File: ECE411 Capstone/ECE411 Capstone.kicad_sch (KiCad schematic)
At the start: 27 parts, among them SW1 SW_Push, SW2 SW_Push, SW3 SW_Push, SW4 SW_Push, SW5 SW_Push, SW6 SW_Push, SW7 SW_Push, U1 IS31FL3218-GR

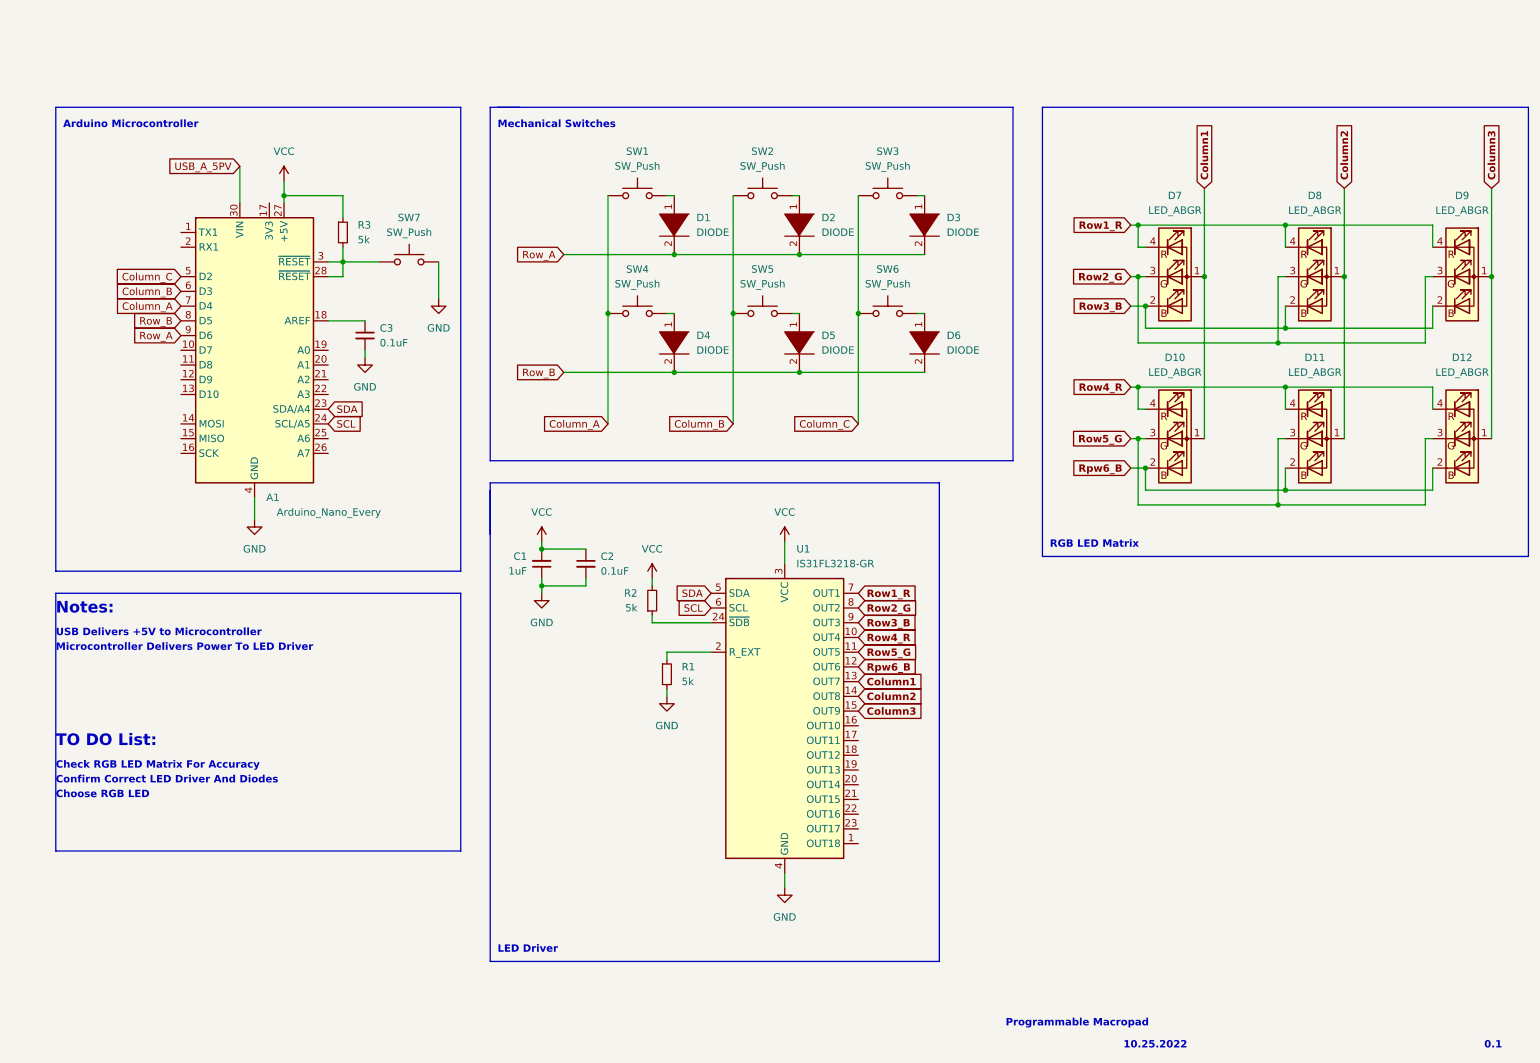
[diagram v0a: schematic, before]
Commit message: Updated Schematic + PCB for review
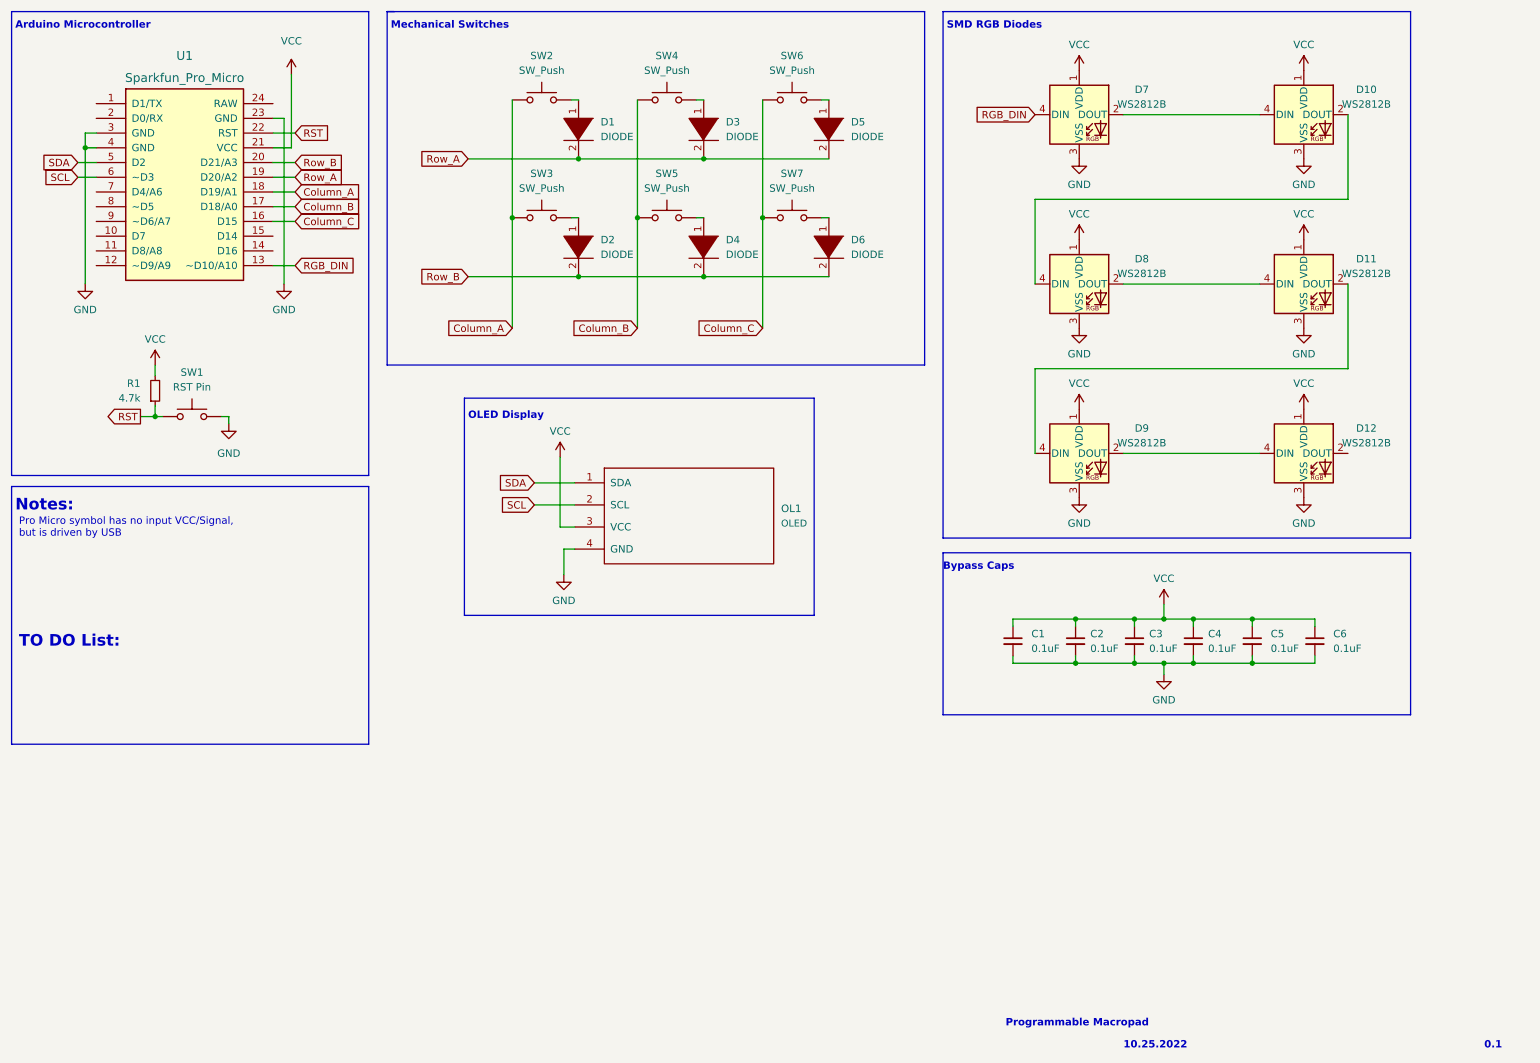
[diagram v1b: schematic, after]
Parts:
- removed A1: Arduino_Nano_Every, Module:Arduino_Nano, symbol MCU_Module:Arduino_Nano_Every
- removed D10, D11, D12, D7, D8, D9: LED_ABGR, symbol Device:LED_ABGR
- removed R2, R3: 5k, symbol Device:R_Small
- removed SW7: SW_Push, symbol Switch:SW_Push
- removed U1: IS31FL3218-GR, Package_SO:SOP-24_7.5x15.4mm_P1.27mm, symbol Driver_LED:IS31FL3218-GR
- added C4, C5, C6: 0.1uF, Capacitor_SMD:C_01005_0402Metric, symbol Device:C_Small
- added D10, D11, D12, D7, D8, D9: WS2812B, LED_SMD:LED_WS2812B_PLCC4_5.0x5.0mm_P3.2mm, symbol LED:WS2812B
- added OL1: OLED, KBD Keyboard stuff:OLED_v2, symbol SSD1306 OLED:OLED
- added SW1: RST Pin, Button_Switch_SMD:SW_Push_1P1T_NO_6x6mm_H9.5mm, symbol Switch:SW_Push
- added U1: Sparkfun_Pro_Micro, KBD Keyboard stuff:ProMicro_v3, symbol Arduino:Sparkfun_Pro_Micro
- C1: value 1uF -> 0.1uF; footprint (none) -> Capacitor_SMD:C_01005_0402Metric
- C2, C3: footprint (none) -> Capacitor_SMD:C_01005_0402Metric
- D1, D6: footprint (none) -> Diode_SMD:D_SOD-123
- D2: renamed from D4; footprint (none) -> Diode_SMD:D_SOD-123
- D3: renamed from D2; footprint (none) -> Diode_SMD:D_SOD-123
- D4: renamed from D5; footprint (none) -> Diode_SMD:D_SOD-123
- D5: renamed from D3; footprint (none) -> Diode_SMD:D_SOD-123
- R1: value 5k -> 4.7k; footprint (none) -> Resistor_SMD:R_0201_0603Metric
- SW2: renamed from SW1; footprint (none) -> Mechanical switches:MXOnly-1U-NoLED
- SW3: renamed from SW4; footprint (none) -> Mechanical switches:MXOnly-1U-NoLED
- SW4: renamed from SW2; footprint (none) -> Mechanical switches:MXOnly-1U-NoLED
- SW5: footprint (none) -> Mechanical switches:MXOnly-1U-NoLED
- SW6: renamed from SW3; footprint (none) -> Mechanical switches:MXOnly-1U-NoLED
- SW7: renamed from SW6; footprint (none) -> Mechanical switches:MXOnly-1U-NoLED
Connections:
- net Column_A: now also U1.18 (D19/A1)
- net Column_B: now also U1.17 (D18/A0)
- net Column_C: now also U1.16 (D15)
- net GND: now also C1.2, C4.2, C5.2, C6.2, D10.3 (VSS), D11.3 (VSS), D12.3 (VSS), D7.3 (VSS), D8.3 (VSS), D9.3 (VSS), OL1.4 (GND), SW1.2, U1.23 (GND), U1.3 (GND), U1.4 (GND); no longer C1.1, R1.2
- net Row_A: now also U1.19 (D20/A2)
- net Row_B: now also U1.20 (D21/A3)
- net SCL: now also OL1.2 (SCL), U1.6 (~D3)
- net SDA: now also OL1.1 (SDA), U1.5 (D2)
- net VCC: now also C1.1, C3.1, R1.2, C4.1, C5.1, C6.1, D10.1 (VDD), D11.1 (VDD), D12.1 (VDD), D7.1 (VDD), D8.1 (VDD), D9.1 (VDD), OL1.3 (VCC), U1.21 (VCC); no longer C1.2
- net RST: now reaches R1.1
- net RST: now also SW1.1, U1.22 (RST)
- new net: D12.4 (DIN), D9.2 (DOUT)
- new net: D11.2 (DOUT), D9.4 (DIN)
- new net: D11.4 (DIN), D8.2 (DOUT)
- new net: D10.2 (DOUT), D8.4 (DIN)
- new net: D10.4 (DIN), D7.2 (DOUT)
- new net RGB_DIN: D7.4 (DIN), U1.13 (~D10/A10)
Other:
- note added: "Bypass Caps"
- note added: "OLED Display"
- note added: "Pro Micro symbol has no input VCC/Signal, but is driven by USB"
- note added: "SMD RGB Diodes"
- note removed: "Check RGB LED Matrix For Accuracy"
- note removed: "Choose RGB LED"
- note removed: "Confirm Correct LED Driver And Diodes"
- note removed: "LED Driver"
- note removed: "Microcontroller Delivers Power To LED Driver"
- note removed: "RGB LED Matrix"
- note removed: "USB Delivers +5V to Microcontroller"
- moved on the sheet: D1, D2, D3, D4, D5, D6, SW2, SW3, SW4, SW5, SW6, SW7
